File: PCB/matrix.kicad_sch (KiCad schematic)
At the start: 27 parts, among them SW10 EC_SW, SW11 EC_SW, SW12 EC_SW, SW13 EC_SW, SW14 EC_SW, SW15 EC_SW, SW16 EC_SW, SW17 EC_SW, SW18 EC_SW, SW19 EC_SW, SW2 EC_SW, SW20 EC_SW, SW21 EC_SW, SW22 EC_SW, SW23 EC_SW, SW24 EC_SW, SW25 EC_SW, SW26 EC_SW, SW27 EC_SW, SW28 EC_SW, SW3 EC_SW, SW4 EC_SW, SW5 EC_SW, SW6 EC_SW, SW7 EC_SW, SW8 EC_SW, SW9 EC_SW

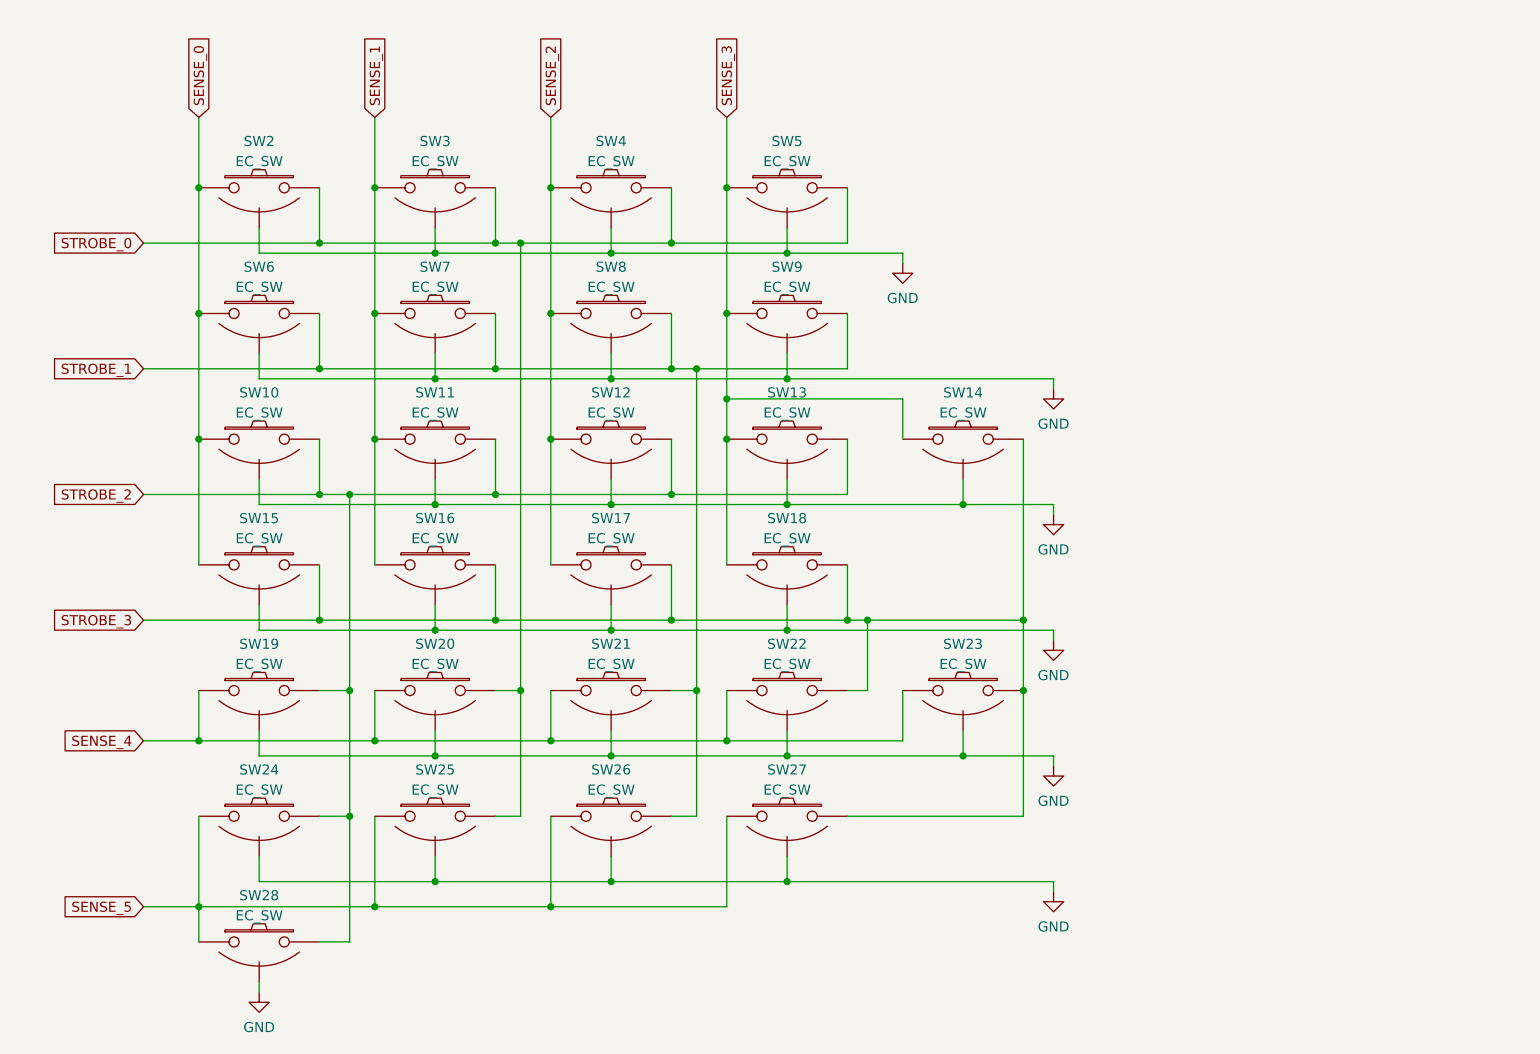
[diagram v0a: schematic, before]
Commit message: First commit, removed unnecessary files, ChatGPT'd the readme, added production and Kicad files for Left&Right sides as well as the Plate.
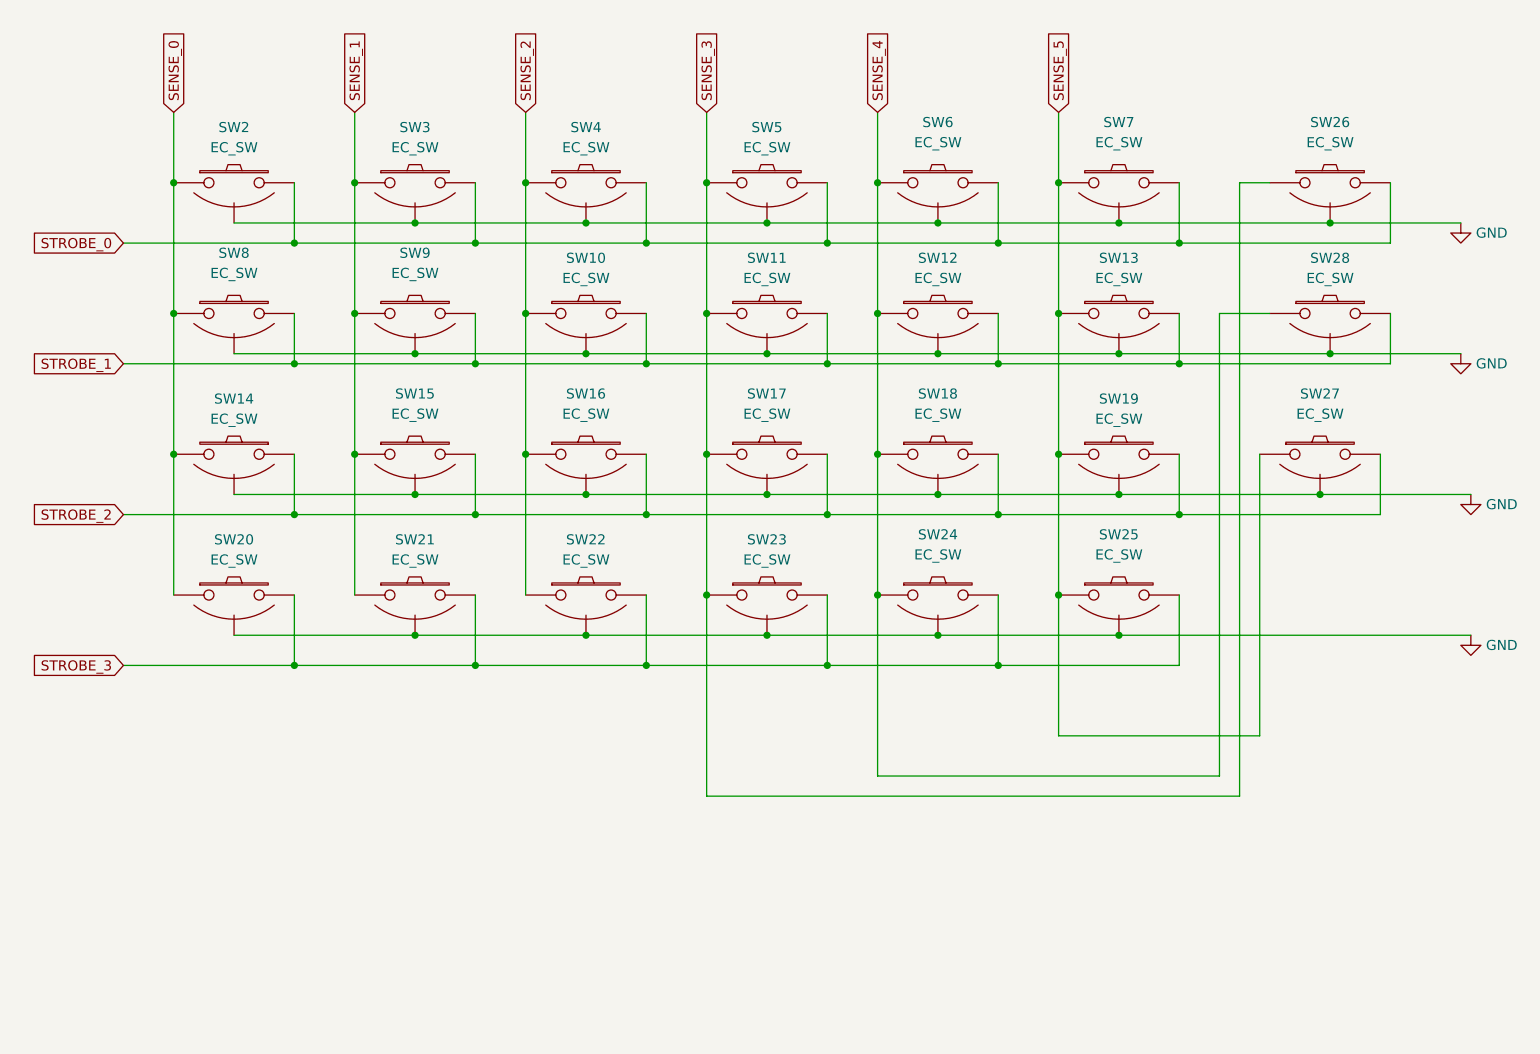
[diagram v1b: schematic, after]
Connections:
- net SENSE_0: now also SW14.2, SW20.1, SW8.1; no longer SW10.1, SW15.1, SW6.1
- net SENSE_1: now also SW15.1, SW21.1, SW9.1; no longer SW11.1, SW16.1, SW7.1
- net SENSE_2: now also SW10.1, SW16.1, SW22.1; no longer SW12.1, SW17.1, SW8.1
- net SENSE_3: now also SW11.1, SW17.1, SW23.1, SW26.1; no longer SW13.1, SW14.2, SW18.1, SW9.1
- net SENSE_4: now also SW12.1, SW18.1, SW24.1, SW28.1, SW6.1; no longer SW19.1, SW20.1, SW21.1, SW22.1, SW23.1
- net SENSE_5: now also SW13.1, SW19.1, SW7.1; no longer SW24.1, SW26.1, SW28.1
- net STROBE_0: now also SW26.2, SW6.2, SW7.2; no longer SW20.2, SW25.2
- net STROBE_1: now also SW10.2, SW11.2, SW12.2, SW13.2, SW28.2; no longer SW21.2, SW26.2, SW6.2, SW7.2
- net STROBE_2: now also SW14.1, SW15.2, SW16.2, SW17.2, SW18.2, SW27.2; no longer SW10.2, SW11.2, SW12.2, SW13.2, SW24.2, SW28.2
- net STROBE_3: now also SW20.2, SW21.2, SW24.2, SW25.2; no longer SW14.1, SW15.2, SW16.2, SW17.2, SW18.2, SW27.2
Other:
- moved on the sheet: SW10, SW11, SW12, SW13, SW14, SW15, SW16, SW17, SW18, SW19, SW2, SW20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
